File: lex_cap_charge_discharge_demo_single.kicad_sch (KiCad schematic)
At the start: 8 parts, among them J1 +5V, J2 GND, SW1 charge, SW2 discharge

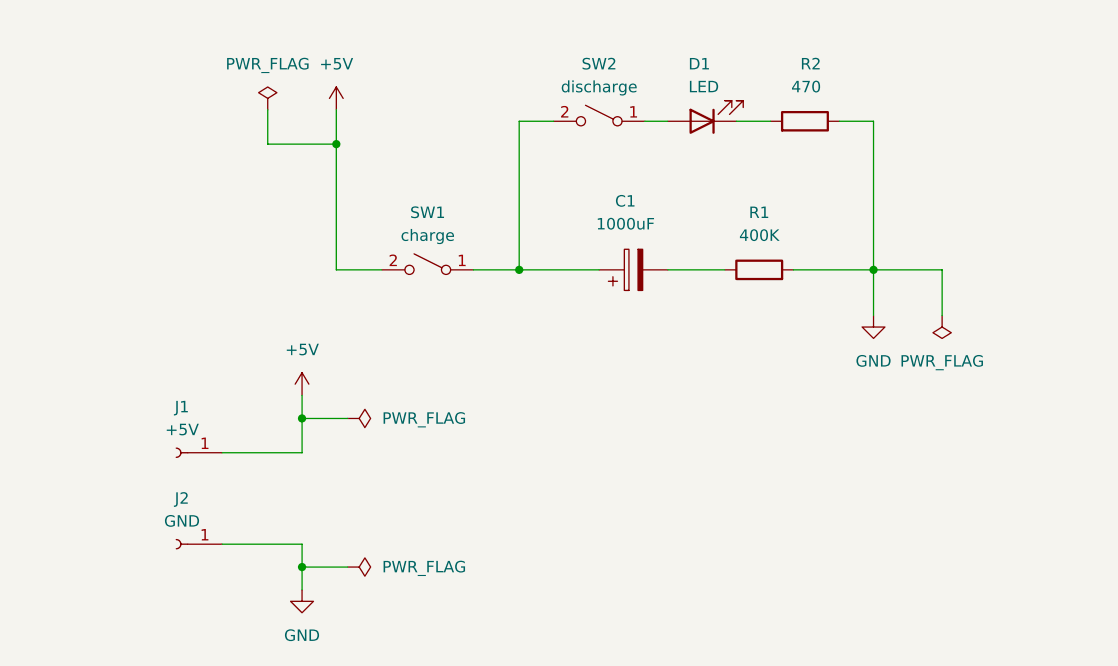
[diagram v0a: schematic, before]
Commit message: put resistor next to +5v, tidy
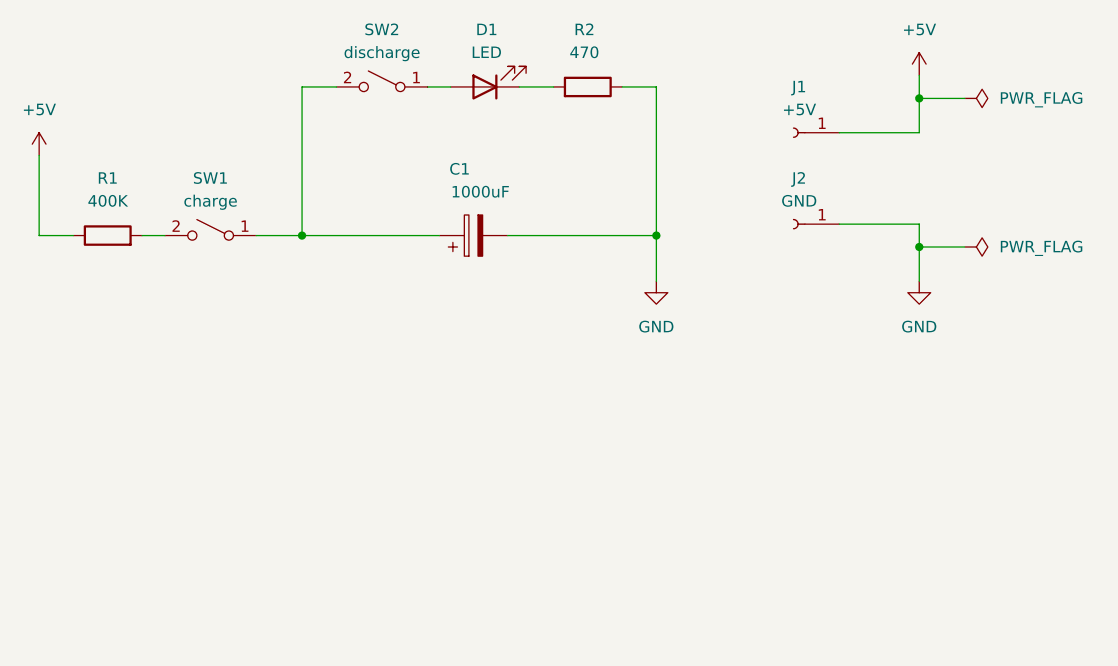
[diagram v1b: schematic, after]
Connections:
- net +5V: now also R1.1; no longer SW1.2 (B)
- net GND: now also C1.2; no longer R1.2
- new net: R1.2, SW1.2 (B)
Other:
- moved on the sheet: C1, D1, J1, J2, R1, R2, SW1, SW2
